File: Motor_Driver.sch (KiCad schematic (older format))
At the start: 16 parts, among them J3 M1, J4 M2, J5 PWR_IN, U1 TB67H420FTG_EL

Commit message: Pre_layout
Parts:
- J3, J4, J5: footprint XT30PB -> Connector_AMASS:AMASS_XT30U-M_1x02_P5.0mm_Vertical
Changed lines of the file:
@@
 F 0 "J3" H 4178 5896 50  0000 L CNN
 F 1 "M1" H 4178 5805 50  0000 L CNN
-F 2 "XT30PB" H 4200 6000 50  0001 L CNN
+F 2 "Connector_AMASS:AMASS_XT30U-M_1x02_P5.0mm_Vertical" H 4200 6000 50  0001 L CNN
 F 3 "https://www.tme.eu/Document/4acc913878197f8c2e30d4b8cdc47230/XT30UPB%20SPEC.pdf" H 4200 5900 50  0001 L CNN
 F 4 "Mini XT60 XT30 Connector for RC Multirotor Racing Drone Quadcopter" H 4200 5800 50  0001 L CNN "Description"
@@
 F 0 "J4" H 4178 6346 50  0000 L CNN
 F 1 "M2" H 4178 6255 50  0000 L CNN
-F 2 "XT30PB" H 4200 6450 50  0001 L CNN
+F 2 "Connector_AMASS:AMASS_XT30U-M_1x02_P5.0mm_Vertical" H 4200 6450 50  0001 L CNN
 F 3 "https://www.tme.eu/Document/4acc913878197f8c2e30d4b8cdc47230/XT30UPB%20SPEC.pdf" H 4200 6350 50  0001 L CNN
 F 4 "Mini XT60 XT30 Connector for RC Multirotor Racing Drone Quadcopter" H 4200 6250 50  0001 L CNN "Description"
@@
 F 0 "J5" H 4178 6846 50  0000 L CNN
 F 1 "PWR_IN" H 4178 6755 50  0000 L CNN
-F 2 "XT30PB" H 4200 6950 50  0001 L CNN
+F 2 "Connector_AMASS:AMASS_XT30U-M_1x02_P5.0mm_Vertical" H 4200 6950 50  0001 L CNN
 F 3 "https://www.tme.eu/Document/4acc913878197f8c2e30d4b8cdc47230/XT30UPB%20SPEC.pdf" H 4200 6850 50  0001 L CNN
 F 4 "Mini XT60 XT30 Connector for RC Multirotor Racing Drone Quadcopter" H 4200 6750 50  0001 L CNN "Description"

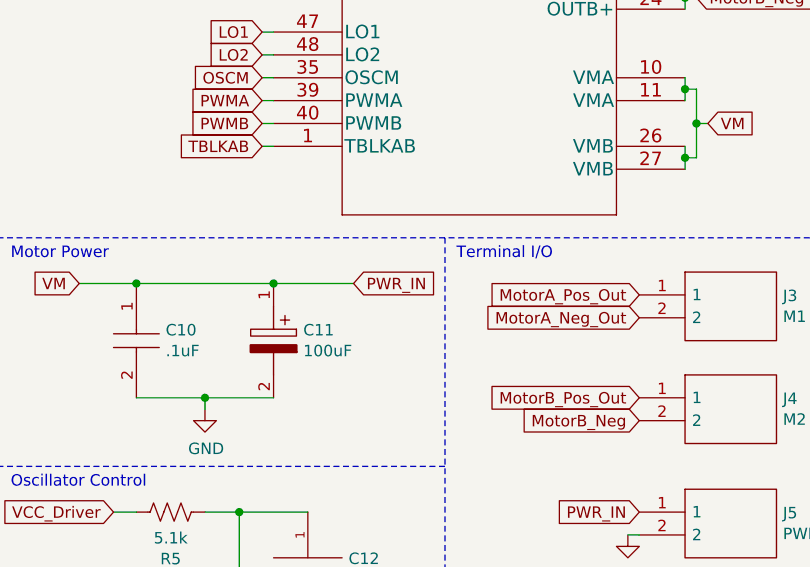
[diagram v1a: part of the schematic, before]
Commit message: Layout Rev_One done pre review
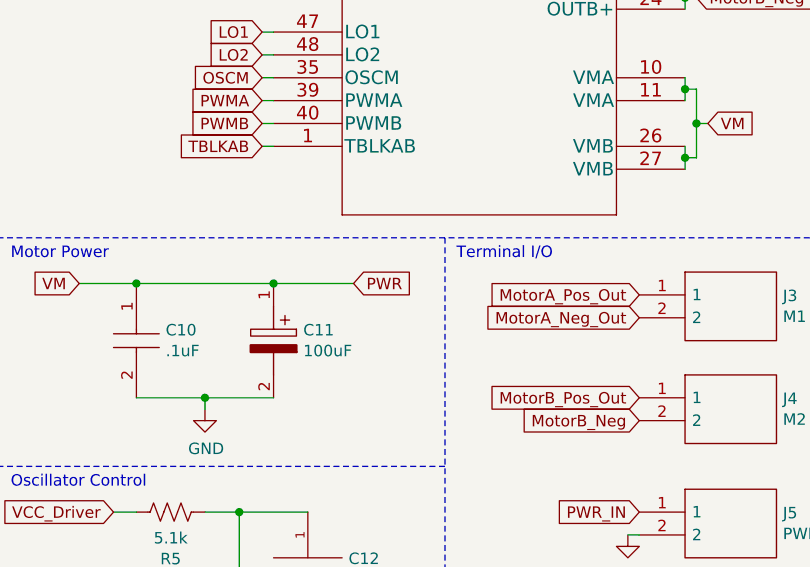
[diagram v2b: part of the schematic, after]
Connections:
- net PWR_IN: no longer C10.1, C11.1, U1.10 (VMA), U1.11 (VMA), U1.26 (VMB), U1.27 (VMB)
- new net PWR: C10.1, C11.1, U1.10 (VMA), U1.11 (VMA), U1.26 (VMB), U1.27 (VMB)
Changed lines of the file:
@@
 	1    0    0    -1
 $EndComp
-Text GLabel 2300 5850 2    50   Input ~ 0
-PWR_IN
 Wire Wire Line
 	3750 3850 3750 3900
@@
 	1    0    0    -1
 $EndComp
+Text GLabel 2300 5850 2    50   Input ~ 0
+PWR
 $EndSCHEMATC
